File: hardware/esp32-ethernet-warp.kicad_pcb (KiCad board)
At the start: 4 copper layers, 104 x 42 mm, 116 parts, among them J201 TJLC_001LA1, P101 FLASH, P201 CON-SENSOR2, P202 CON-SENSOR2, P205 CON-SENSOR2, P206 CON-SENSOR2, Q101 BC817, Q102 BC817, SW101 B3U-1000P, SW102 B3U-1000P, U101 TMP1075NDRLR, U103 PCF8523T, U104 ESP32-WROVER-E, U106 171010502, U201 74AHC244, U203 74AHC244, U301 KSZ8091RNACA, U302 SN74LV138APW, X101 32.768kHz, X301 25Mhz-10pF

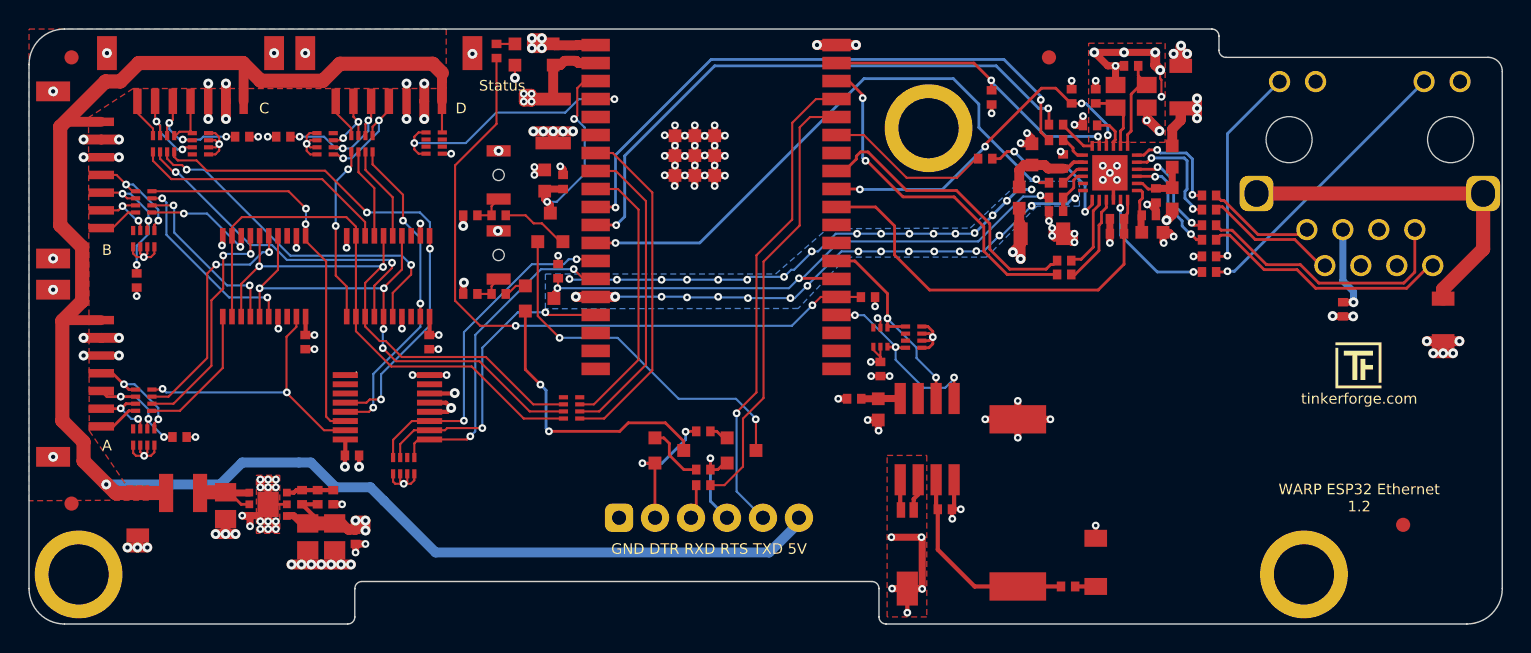
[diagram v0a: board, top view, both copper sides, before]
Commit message: version 1.3 finished
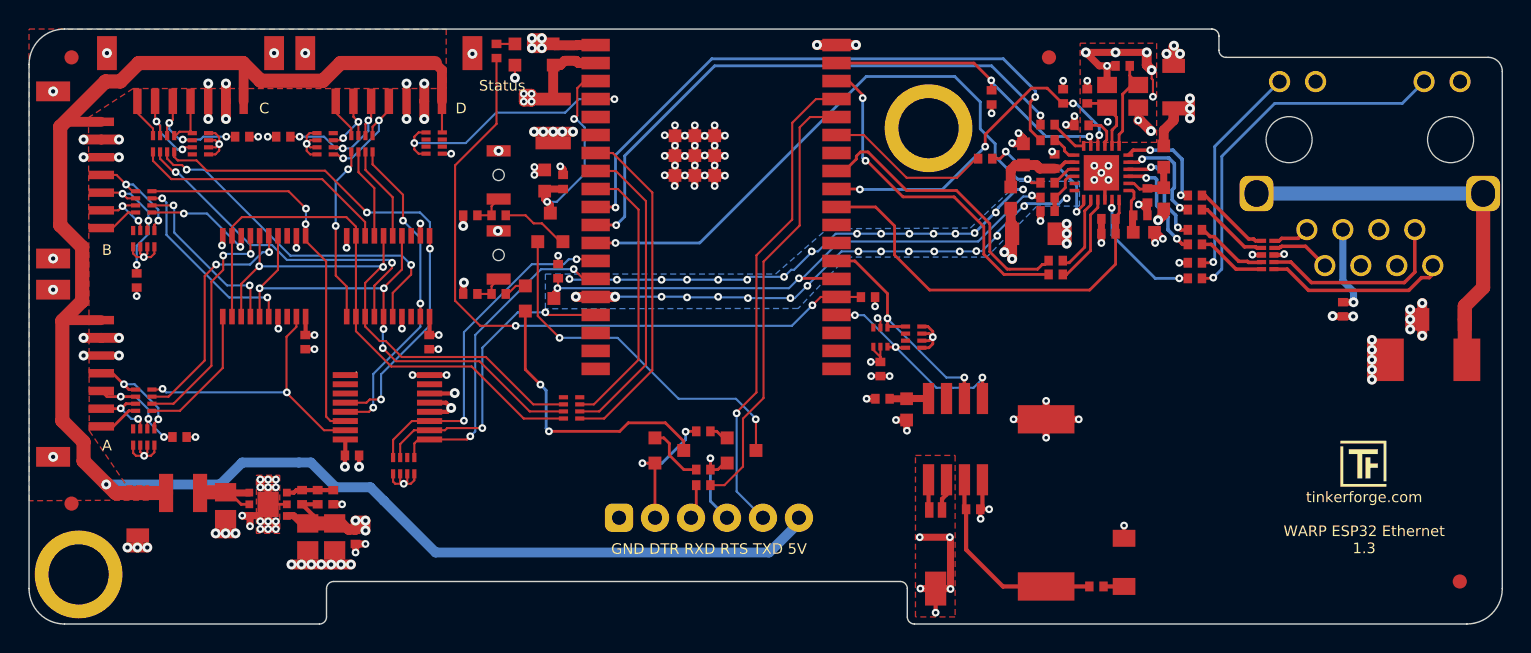
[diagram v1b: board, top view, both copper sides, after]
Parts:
- removed F101: DRILL, kicad-libraries:LSMTSO-M3
- added R203: DNP, kicad-libraries:1812, F.Cu at (252.6, 39.6)
- added U202: TPD4S010DQA, kicad-libraries:TPD4S010DQA, F.Cu at (241.2, 32.2)
- C312: value 100nF -> 100nF/50V
- L101: value NR3015T6R8M -> NR3015T1R5N
- moved G*** 6.96 mm to (247.9, 47.0)
- moved Fiducial_Mark 5.66 mm to (254.8, 55.3)
- moved C102 2.00 mm to (225.6, 49.8)
- moved C104 2.00 mm to (220.4, 50.2)
- moved C107 2.00 mm to (215.7, 43.1)
- moved D102 2.00 mm to (231.1, 54.0)
- moved R101 2.00 mm to (229.1, 55.6)
- moved R103 2.00 mm to (214.0, 42.4)
- moved U103 2.00 mm to (219.2, 45.2)
- moved X101 2.00 mm to (217.8, 55.8)
- moved R315 1.10 mm to (236.1, 32.8)
- moved R316 1.10 mm to (236.1, 33.9)
- moved R313 1.05 mm to (236.1, 30.5)
- moved R314 1.05 mm to (236.1, 31.5)
- moved R311 1.00 mm to (236.1, 28.1)
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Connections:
- net Net-(J201-RD+) renamed RXIPx
- net Net-(J201-RD-) renamed RXINx
- net Net-(J201-TD1+) renamed TXOPx
- net Net-(J201-TD1-) renamed TXONx
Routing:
- net 3V3: track 67.4 -> 90.0 mm
- net GND: track 252.1 -> 266.1 mm, vias 195 -> 201
- net Net-(J201-Pad11): track 20.2 -> 26.0 mm
- net SHD: track 24.6 -> 28.4 mm
- net SCL: track 15.3 -> 17.0 mm
- net SDA: track 14.1 -> 15.8 mm
- net RMII_RXD1: track 41.5 -> 40.7 mm
- net Net-(J201-Pad9): track 14.6 -> 15.4 mm
- net ESP_IO0: track 41.7 -> 41.1 mm
- net RMII_MDC: track 22.7 -> 22.1 mm
- net RMII_RESET: track 29.3 -> 28.7 mm
- net TXON: track 8.12 -> 7.56 mm
- net TXOPx: track 7.69 -> 8.22 mm
- net RMII_TXD0: track 21.0 -> 20.5 mm
- net RXIP: track 7.37 -> 7.88 mm
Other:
- outline, holes or cut-outs redrawn
- board text added: "WARP ESP32 Ethernet 1.3"
- board text removed: "WARP ESP32 Ethernet 1.2"

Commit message: Revert "version 1.3 finished"
This reverts commit c7f26ed94f03ba8104635e5142b3afb52f15755f.
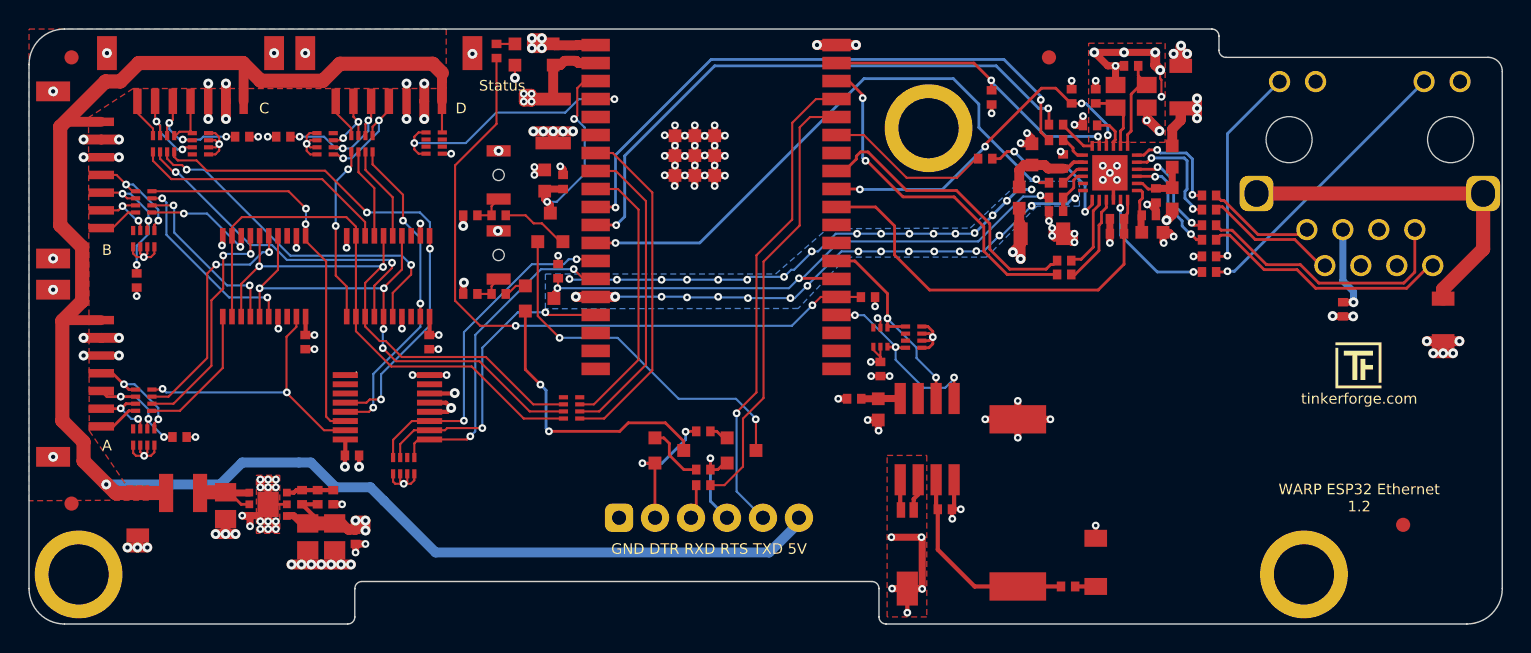
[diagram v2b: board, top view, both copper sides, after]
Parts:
- removed R203: DNP, kicad-libraries:1812
- removed U202: TPD4S010DQA, kicad-libraries:TPD4S010DQA
- added F101: DRILL, kicad-libraries:LSMTSO-M3, F.Cu at (243.8, 54.8)
- C312: value 100nF/50V -> 100nF
- L101: value NR3015T1R5N -> NR3015T6R8M
- moved G*** 6.96 mm to (247.6, 40.0)
- moved Fiducial_Mark 5.66 mm to (250.8, 51.3)
- moved C102 2.00 mm to (223.6, 49.8)
- moved C104 2.00 mm to (218.4, 50.2)
- moved C107 2.00 mm to (213.7, 43.1)
- moved D102 2.00 mm to (229.1, 54.0)
- moved R101 2.00 mm to (227.1, 55.6)
- moved R103 2.00 mm to (212.0, 42.4)
- moved U103 2.00 mm to (217.2, 45.2)
- moved X101 2.00 mm to (215.8, 55.8)
- moved R315 1.10 mm to (237.1, 32.4)
- moved R316 1.10 mm to (237.1, 33.5)
- moved R313 1.05 mm to (237.1, 30.1)
- moved R314 1.05 mm to (237.1, 31.2)
- moved R311 1.00 mm to (237.1, 28.1)
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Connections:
- net RXINx renamed Net-(J201-RD-)
- net RXIPx renamed Net-(J201-RD+)
- net TXONx renamed Net-(J201-TD1-)
- net TXOPx renamed Net-(J201-TD1+)
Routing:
- net 3V3: track 90.0 -> 67.4 mm
- net GND: track 266.1 -> 252.1 mm, vias 201 -> 195
- net Net-(J201-Pad11): track 26.0 -> 20.2 mm
- net SHD: track 28.4 -> 24.6 mm
- net SCL: track 17.0 -> 15.3 mm
- net SDA: track 15.8 -> 14.1 mm
- net RMII_RXD1: track 40.7 -> 41.5 mm
- net Net-(J201-Pad9): track 15.4 -> 14.6 mm
- net ESP_IO0: track 41.1 -> 41.7 mm
- net RMII_MDC: track 22.1 -> 22.7 mm
- net RMII_RESET: track 28.7 -> 29.3 mm
- net TXON: track 7.56 -> 8.12 mm
- net Net-(J201-TD1+): track 8.22 -> 7.69 mm
- net RMII_TXD0: track 20.5 -> 21.0 mm
- net RXIP: track 7.88 -> 7.37 mm
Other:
- outline, holes or cut-outs redrawn
- board text added: "WARP ESP32 Ethernet 1.2"
- board text removed: "WARP ESP32 Ethernet 1.3"
